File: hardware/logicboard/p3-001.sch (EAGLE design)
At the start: 27 parts, among them IC1 74LS07N, IC2 LTC485N, IC3 LTC485N

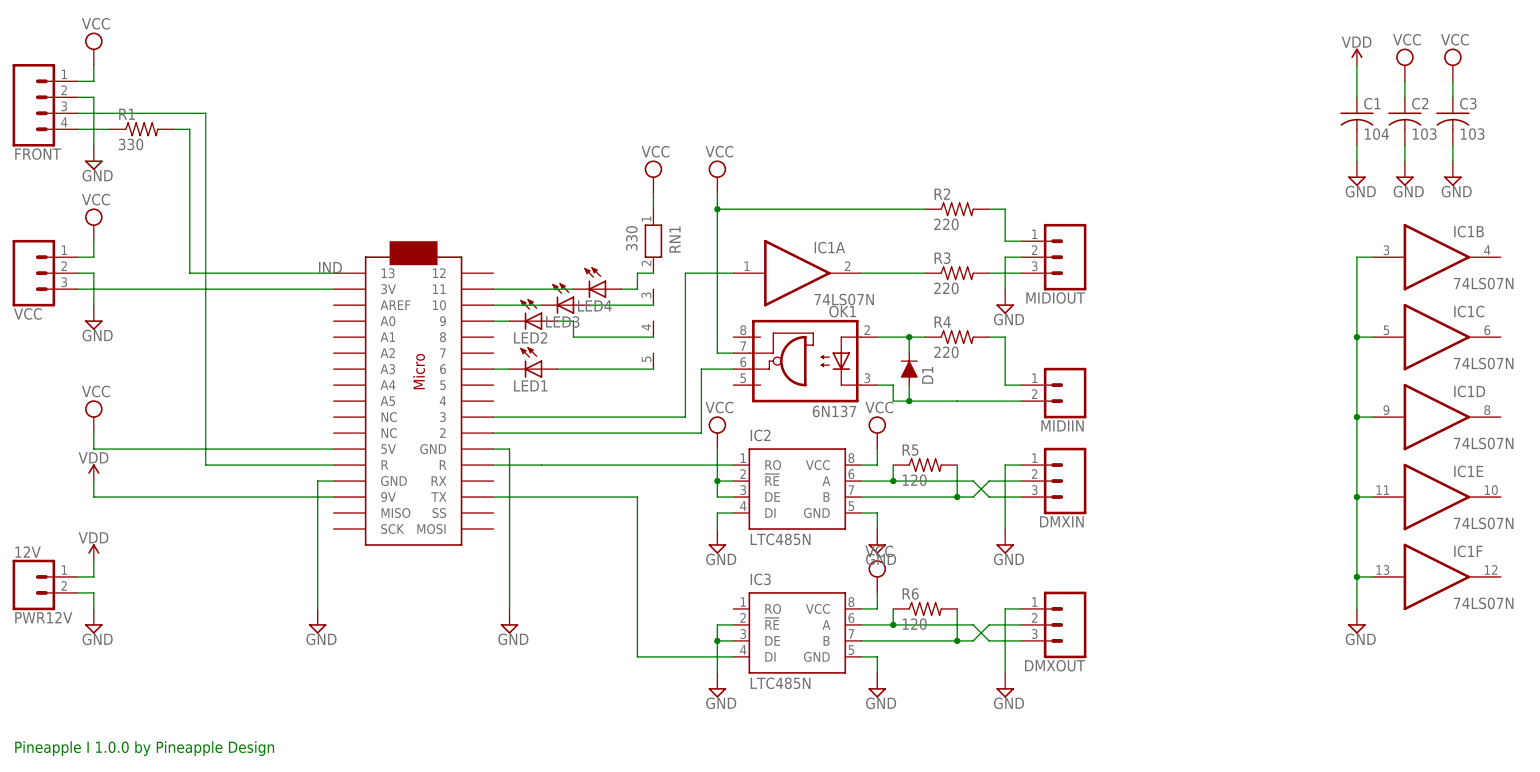
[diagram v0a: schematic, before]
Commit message: DIP SW.
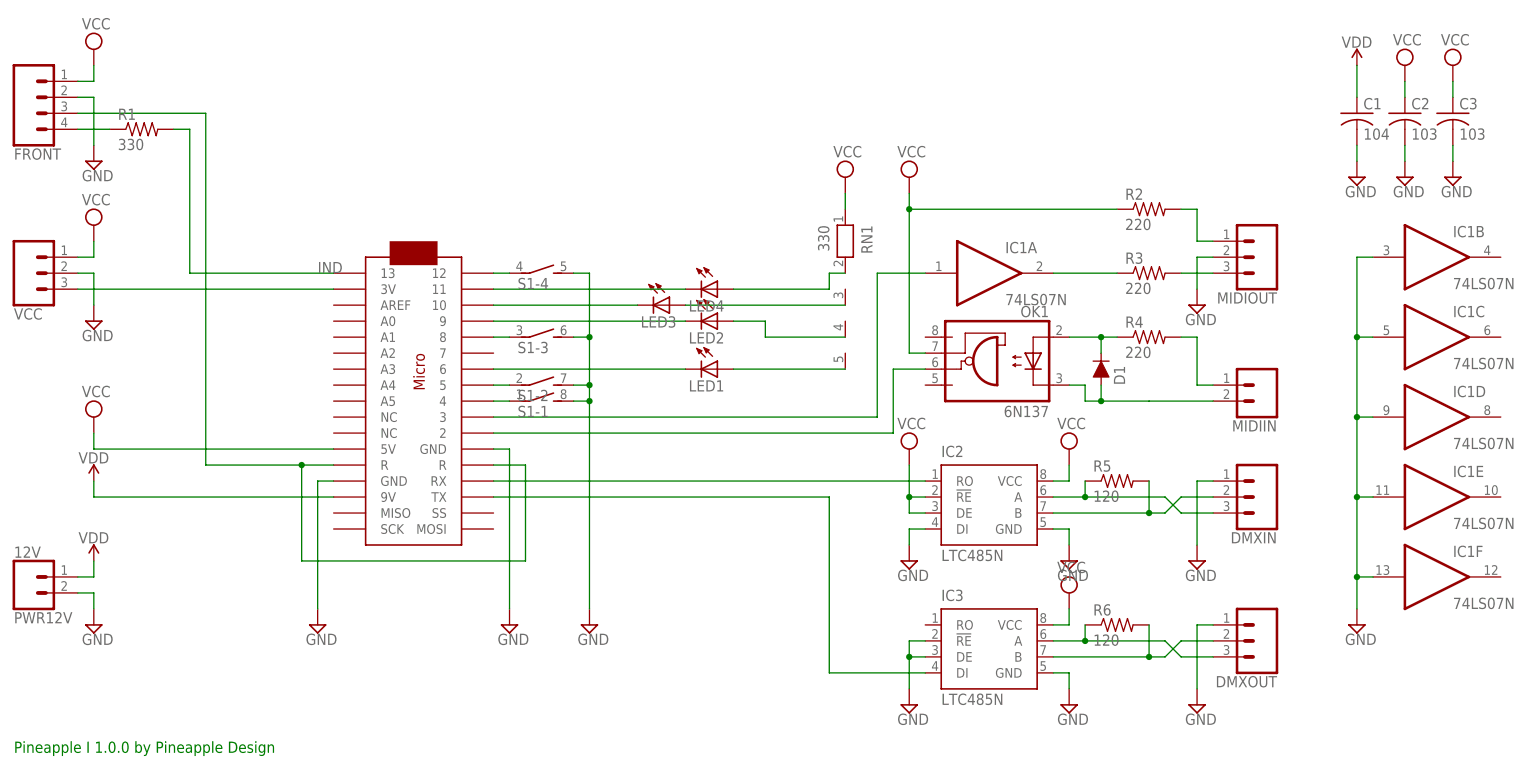
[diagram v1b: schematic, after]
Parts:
- added S1: (no value), switch-dil:DIP04S
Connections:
- new net N$19: S1-1.1, U$1.4
- new net N$20: S1-2.1, U$1.5
- new net N$21: S1-3.1, U$1.8
- new net N$22: S1-4.1, U$1.12
- net GND: now also S1-1.2, S1-2.2, S1-3.2, S1-4.2
- net N$10: now also U$1.RX; no longer U$1.R@2
- net RST: now also U$1.R@2
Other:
- moved on the sheet: D1, DMXIN, DMXOUT, IC1A, IC2, IC3, LED1, LED2, LED3, LED4, MIDIIN, MIDIOUT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
